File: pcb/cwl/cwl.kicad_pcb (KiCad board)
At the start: 2 copper layers, 60.5 x 62 mm, 25 parts, among them J1 UEXT, J2 OpenTherm, J3 OLED_SH1106, J4 EXT_GPIO, J5 AUX, Q1 2N7002, SW1 EC12E24204A9, U1 LTV-817S-B, U2 LTV-817S-B

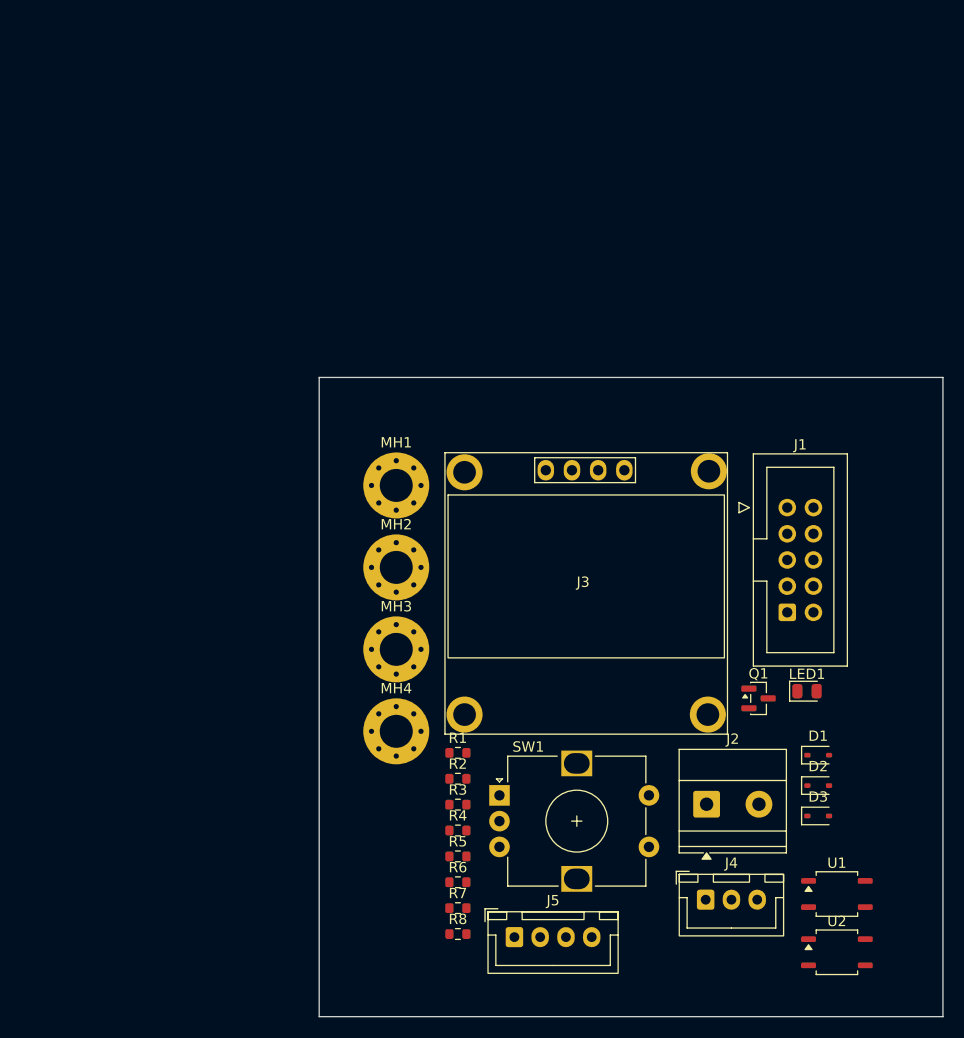
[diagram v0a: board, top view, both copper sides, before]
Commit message: pcb
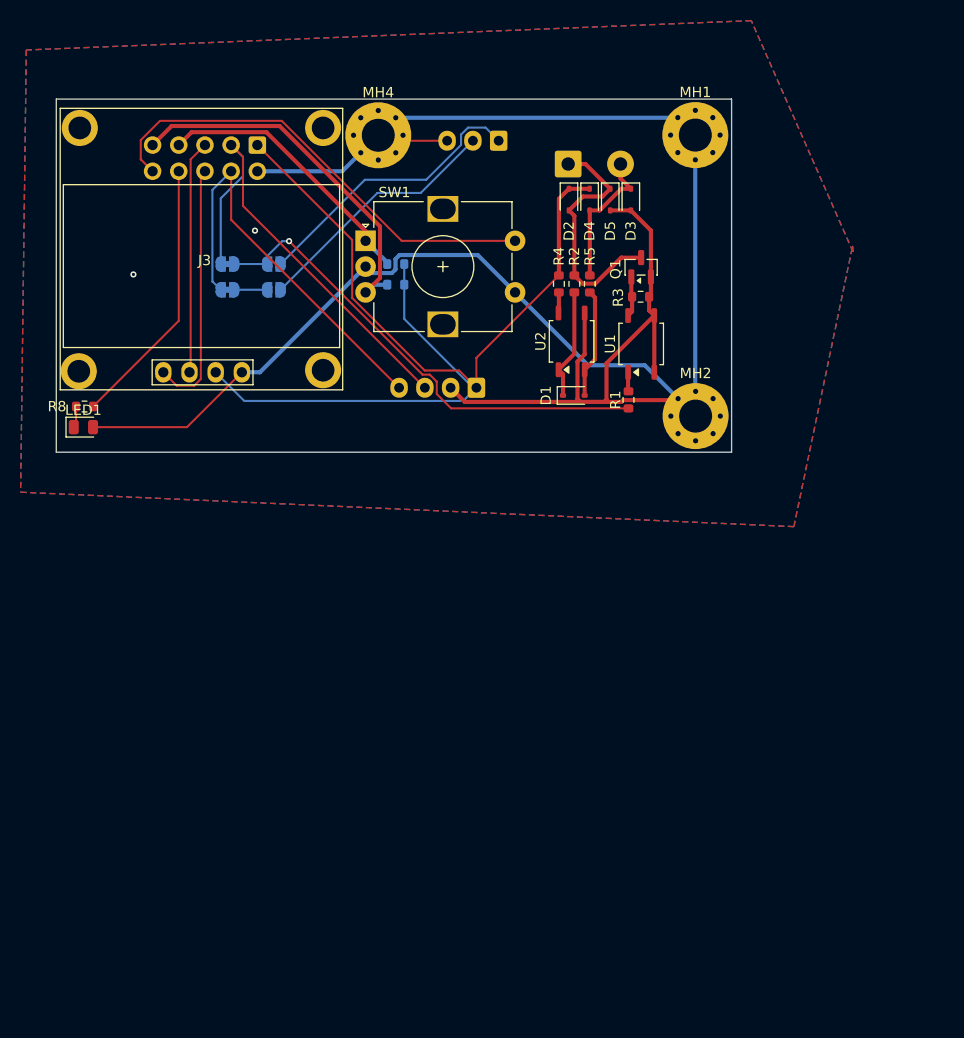
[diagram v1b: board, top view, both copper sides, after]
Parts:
- removed MH3: M3, MountingHole:MountingHole_3.2mm_M3_Pad_Via
- added D4: 1N4148WS, Diode_SMD:D_SOD-323, F.Cu at (123.7, 50.2)
- added D5: 1N4148WS, Diode_SMD:D_SOD-323, F.Cu at (125.7, 50.2)
- added SB1: GPIO4→OT_TX, Jumper:SolderJumper-2_P1.3mm_Open_RoundedPad1.0x1.5mm, B.Cu at (93.1, 56.5)
- added SB2: GPIO36→OT_RX, Jumper:SolderJumper-2_P1.3mm_Open_RoundedPad1.0x1.5mm, B.Cu at (93.1, 59.0)
- added SB3: TXD→OT_TX, Jumper:SolderJumper-2_P1.3mm_Bridged_RoundedPad1.0x1.5mm, B.Cu at (88.6, 56.5)
- added SB4: RXD→OT_RX, Jumper:SolderJumper-2_P1.3mm_Bridged_RoundedPad1.0x1.5mm, B.Cu at (88.6, 59.0)
- D1: value BZX384-C3V3 -> BZX384-C4V7
- J1, J2, J4, J5, R6, R7: moved to B.Cu
- moved J4 76.3 mm to (114.9, 44.5), turned to 180 degrees
- moved LED1 74.7 mm to (74.6, 72.3)
- moved J1 70.9 mm to (81.3, 45.0), turned to -90 degrees
- moved U2 64.6 mm to (122.0, 64.0), turned to 90 degrees
- moved J2 63.5 mm to (121.6, 46.8)
- moved R8 62.7 mm to (74.7, 70.3), turned to 180 degrees
- moved D3 62.5 mm to (127.7, 50.2), turned to -90 degrees
- moved D2 61.8 mm to (121.7, 50.2), turned to -90 degrees
- moved R7 60.8 mm to (104.9, 58.5)
- moved R6 60.3 mm to (104.9, 56.5)
- moved MH4 57.8 mm to (103.2, 44.0)
- moved R5 57.0 mm to (123.8, 58.4), turned to 90 degrees
- moved U1 56.6 mm to (128.7, 64.2), turned to 90 degrees
- moved SW1 55.3 mm to (102.0, 54.2)
- moved R4 53.9 mm to (120.8, 58.4), turned to 90 degrees
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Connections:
- J4 pad 1: GPIO4_OT_TX -> GPIO4
- J4 pad 2: GPIO36_OT_RX -> GPIO36
- R1 pad 1: GPIO4_OT_TX -> OT_TX_SIG
- R4 pad 1: GPIO36_OT_RX -> OT_RX_SIG
- U2 pad 4: GPIO36_OT_RX -> OT_RX_SIG
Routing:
- net GND: track 0.00 -> 215.6 mm, vias 0 -> 2
- net +3V3: track 0.00 -> 101.4 mm
- net OT_TX_SIG: track 0.00 -> 47.0 mm, vias 0 -> 1
- net ENC_SW: track 0.00 -> 45.4 mm
- net UEXT_TXD: track 0.00 -> 44.2 mm
- net UEXT_RXD: track 0.00 -> 40.3 mm
- net ENC_DT: track 0.00 -> 36.3 mm
- net GPIO4: track 0.00 -> 27.8 mm
- net ENC_CLK: track 0.00 -> 27.5 mm
- net LED_GPIO: track 0.00 -> 26.3 mm
- net SDA: track 0.00 -> 24.8 mm
- net GPIO36: track 0.00 -> 24.6 mm
- net OT+: track 0.00 -> 24.3 mm
- net SCL: track 0.00 -> 22.7 mm
- net OT-: track 0.00 -> 14.0 mm
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- added copper zone on B.Cu, net GND
- added copper zone on F.Cu, net GND
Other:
- board size 60.5 x 62 mm -> 65.5 x 34.2 mm
